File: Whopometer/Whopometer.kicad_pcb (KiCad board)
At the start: 2 copper layers, 62 x 22.5 mm, 50 parts, among them J1 USB_B_Micro, J2 Conn_01x04_Socket, J3 Micro_SD_Card, J4 Conn_01x02_Socket, SW1 SW_SPDT, U1 H3LIS331DLTR, U2 STM32F103C8Tx, U3 AMS1117-3.3, U4 W25Q128JVS, Y1 16MHz

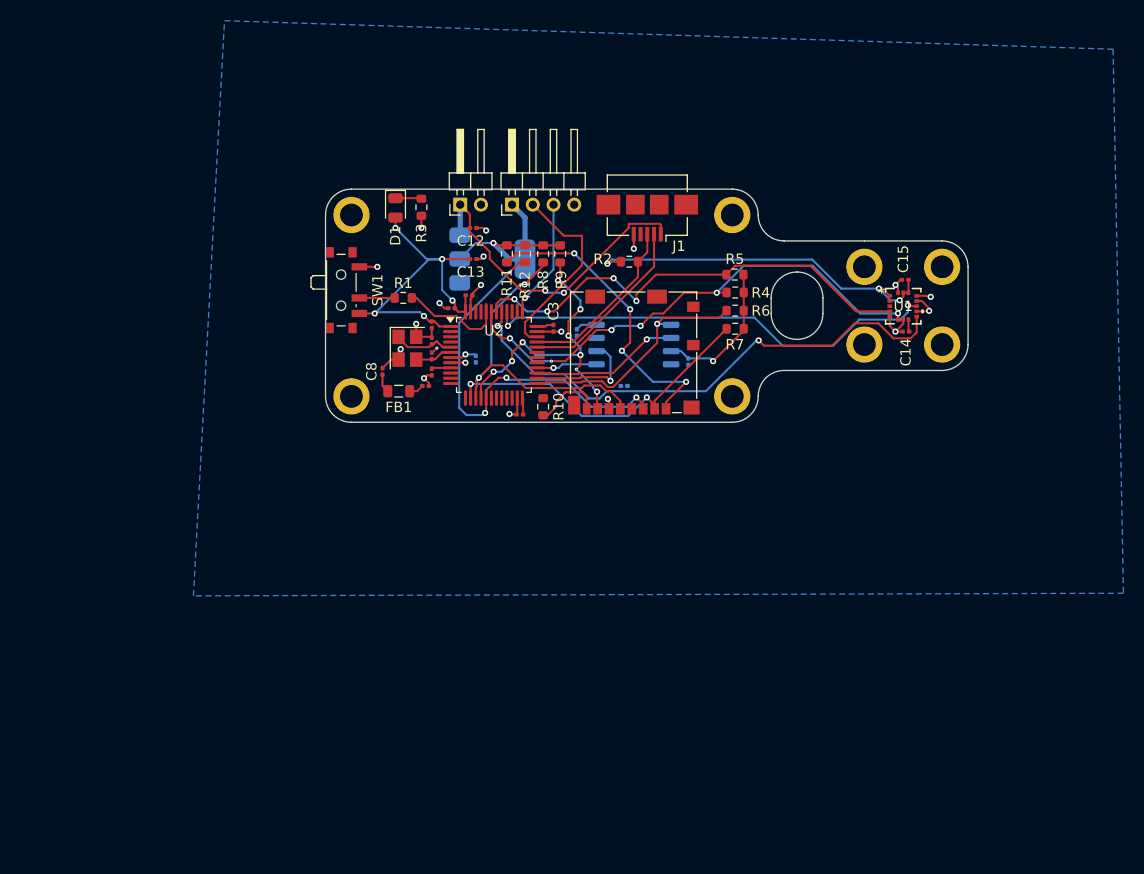
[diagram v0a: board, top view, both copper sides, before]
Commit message: pls
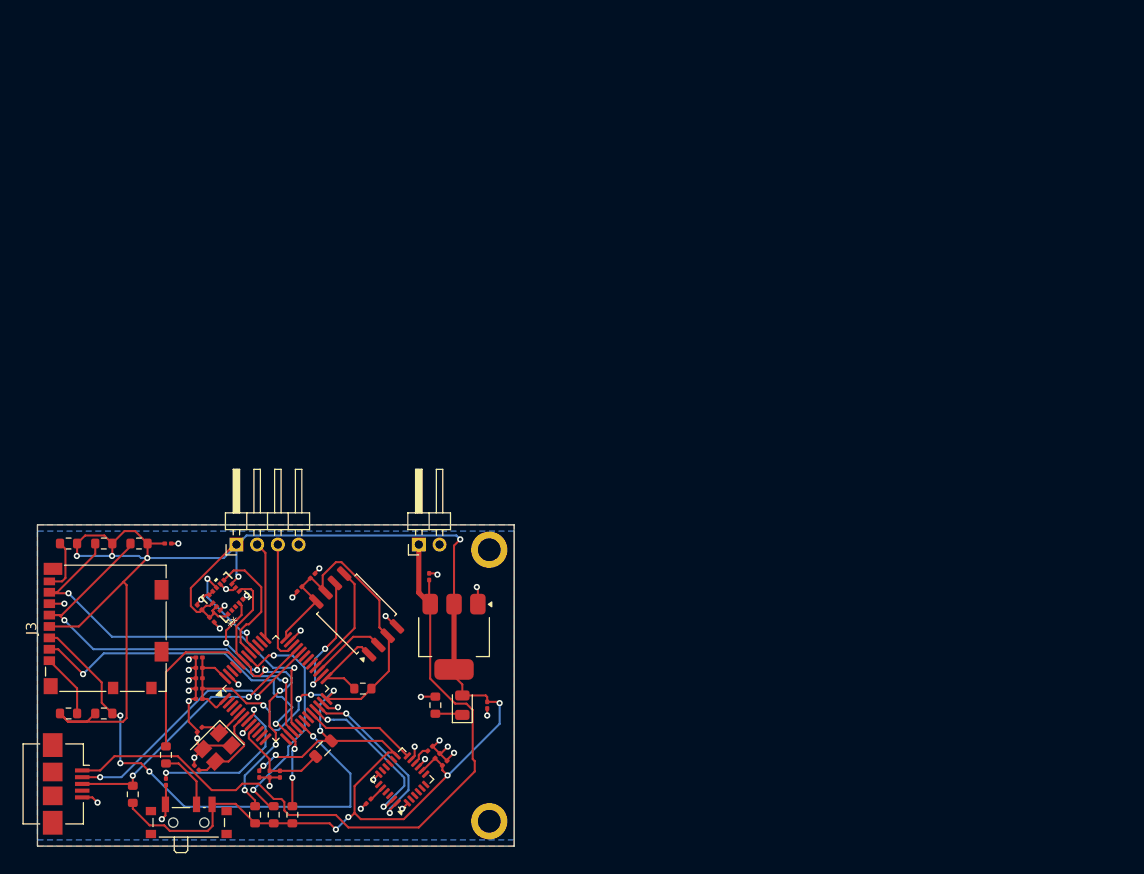
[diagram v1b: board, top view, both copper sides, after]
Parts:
- removed H3, H4, H5, H6, H7, H8: MountingHole, MountingHole:MountingHole_2.2mm_M2_ISO7380_Pad
- added C21: 0.1u, Capacitor_SMD:C_0201_0603Metric, F.Cu at (132.1, 133.0)
- added C22: 2200pF, Capacitor_SMD:C_0201_0603Metric, F.Cu at (126.1, 138.1)
- added C23: 0.1u, Capacitor_SMD:C_0201_0603Metric, F.Cu at (132.8, 133.7)
- added C24: 0.01uF, Capacitor_SMD:C_0201_0603Metric, F.Cu at (133.5, 134.4)
- added U6: MPU-6050, Sensor_Motion:InvenSense_QFN-24_4x4mm_P0.5mm, F.Cu at (129.4, 136.0)
- C16, C17, C18, C9, U3, U4: moved to F.Cu
- moved J1 78.3 mm to (97.0, 136.4), turned to -90 degrees
- moved C15 74.5 mm to (111.0, 120.6), turned to -45 degrees
- moved C14 73.2 mm to (109.8, 119.4), turned to 135 degrees
- moved U1 71.1 mm to (112.4, 118.4), turned to 135 degrees
- moved R2 70.3 mm to (103.4, 137.4), turned to 90 degrees
- moved R5 68.5 mm to (117.0, 139.4), turned to 90 degrees
- moved R4 68.5 mm to (115.2, 139.4), turned to 90 degrees
- moved R7 63.4 mm to (118.8, 139.4), turned to 90 degrees
- moved R11 61.3 mm to (97.2, 129.6), turned to 0 degrees
- moved R12 60.2 mm to (100.6, 129.6), turned to 0 degrees
- moved H2 60.0 mm to (137.8, 140.0)
- moved J3 57.5 mm to (100.8, 121.4), turned to 90 degrees
- moved SW1 53.2 mm to (108.8, 139.8), turned to 0 degrees
- moved R9 52.2 mm to (100.6, 113.2), turned to 0 degrees
- moved R6 51.2 mm to (125.6, 127.2)
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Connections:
- J2 pad 2: /SWDIO -> /SWCLCK
- J2 pad 3: /SWCLCK -> /SWDIO
- U2 pad 20: unconnected-(U2-PB2-Pad20) -> /INT_3
- U2 pad 21: unconnected-(U2-PB10-Pad21) -> /I2C2_SCL
- U2 pad 22: unconnected-(U2-PB11-Pad22) -> /I2C2_SDA
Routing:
- net +3.3V: track 114.9 -> 268.2 mm, vias 10 -> 16
- net VBUS: track 31.2 -> 71.7 mm, vias 2 -> 0
- net /INT_2: track 51.5 -> 12.4 mm, vias 2 -> 0
- net /INT_1: track 44.4 -> 10.1 mm
- net Net-(J3-DAT2): track 29.7 -> 6.20 mm, vias 4 -> 0
- net GND: track 36.3 -> 57.2 mm, vias 19 -> 36
- net /I2C1_SDA: track 49.5 -> 31.3 mm, vias 6 -> 4
- net /I2C2_SDA: track 0.00 -> 17.0 mm, vias 0 -> 2
- net /I2C2_SCL: track 0.00 -> 16.4 mm, vias 0 -> 2
- net /SPI2_CS: track 24.1 -> 8.74 mm, vias 1 -> 0
- net /NRST: track 2.59 -> 16.6 mm, vias 1 -> 2
- net /I2C1_SCL: track 45.3 -> 32.7 mm
- net /INT_3: track 0.00 -> 10.9 mm
- net /USB_D+: track 16.8 -> 26.9 mm, vias 0 -> 2
- net /SPI1_MOSI: track 40.0 -> 49.6 mm
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- added copper zone on F.Cu, net +3.3V
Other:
- board size 62 x 22.5 mm -> 46 x 31 mm
- board text removed: "Whopometer"
